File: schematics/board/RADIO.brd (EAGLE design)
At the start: 76 x 76 mm, 50 parts, among them J1 IPX-RADIO, J2 IPX-ANT

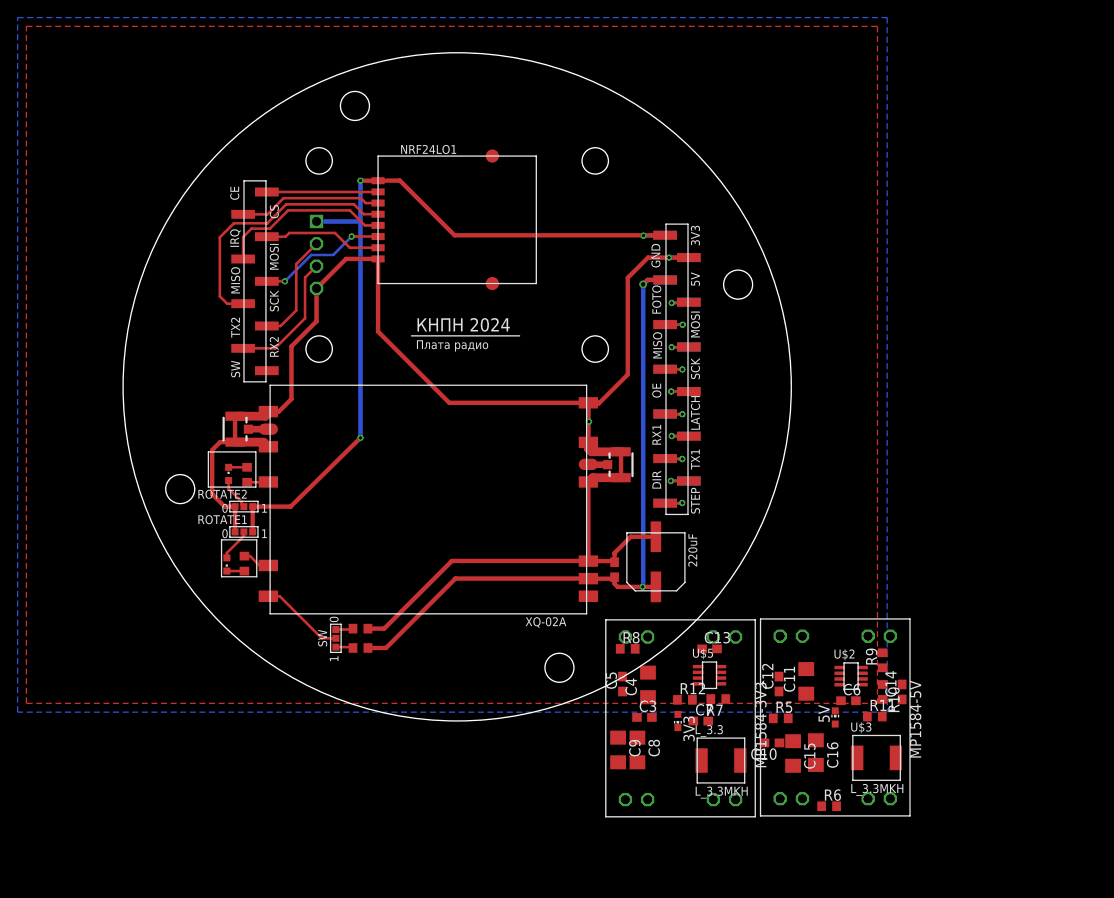
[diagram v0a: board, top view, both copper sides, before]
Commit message: дс дс
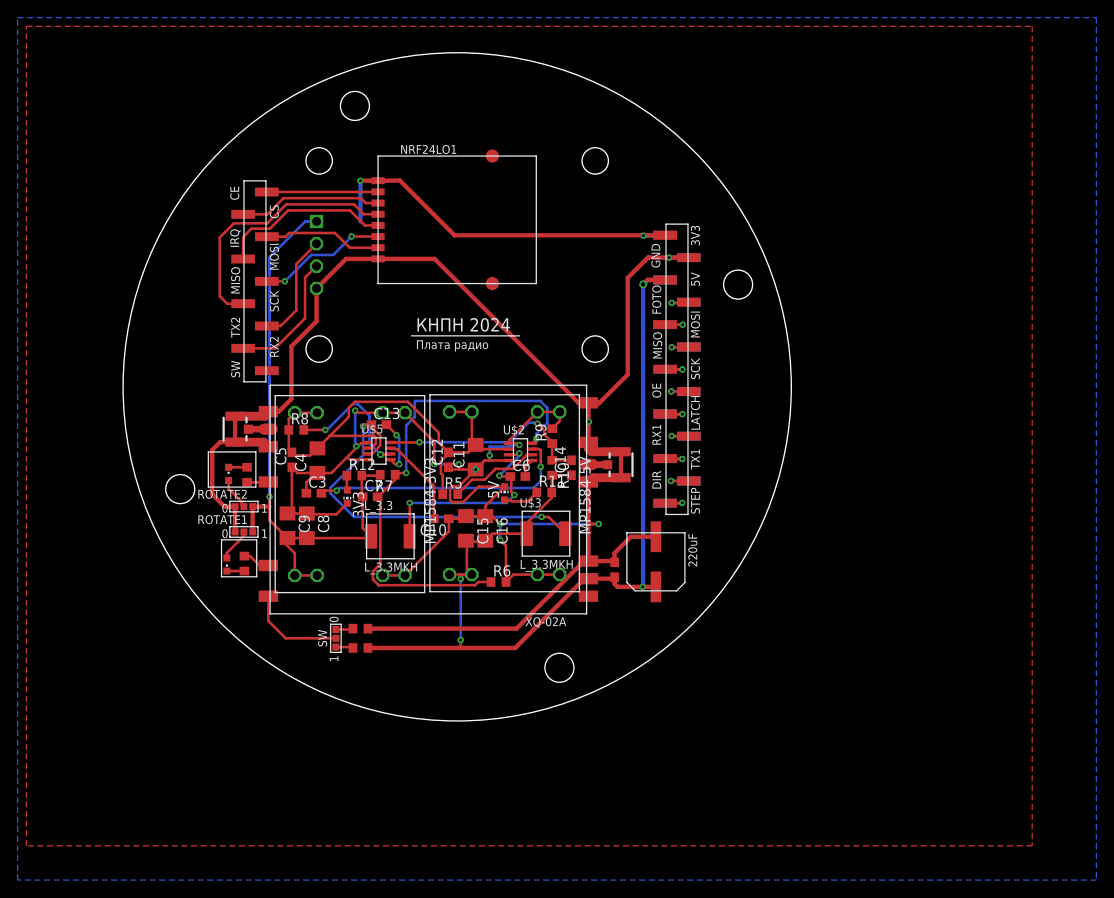
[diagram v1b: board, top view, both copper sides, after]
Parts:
- moved MP1584-3V3 45.4 mm to (37.8, 37.8)
- moved R10 45.4 mm to (60.8, 40.8)
- moved R12 45.4 mm to (38.3, 39.9)
- moved R9 45.4 mm to (60.8, 44.4)
- moved 3V3 45.4 mm to (37.5, 37.5)
- moved 5V 45.4 mm to (55.4, 37.9)
- moved C10 45.4 mm to (48.2, 35.0)
- moved C11 45.4 mm to (52.1, 42.0)
- moved C12 45.4 mm to (49.0, 41.7)
- moved C13 45.4 mm to (41.1, 45.7)
- moved C16 45.4 mm to (53.2, 33.9)
- moved C3 45.4 mm to (33.7, 37.9)
- moved C4 45.4 mm to (34.1, 41.6)
- moved C5 45.4 mm to (31.2, 41.7)
- moved C6 45.4 mm to (56.9, 39.8)
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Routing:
- net GND: track 181.9 -> 309.0 mm, vias 2 -> 12
- net BUS+: track 0.00 -> 57.5 mm
- net N$13: track 0.00 -> 56.6 mm, vias 0 -> 2
- net N$17: track 0.00 -> 43.4 mm, vias 0 -> 2
- net 5V: track 76.8 -> 108.0 mm, vias 2 -> 4
- net N$9: track 0.00 -> 30.1 mm, vias 0 -> 2
- net N$18: track 0.00 -> 24.8 mm, vias 0 -> 2
- net N$12: track 0.00 -> 24.4 mm, vias 0 -> 4
- net 3V3: track 92.3 -> 114.9 mm
- net N$15: track 0.00 -> 15.3 mm, vias 0 -> 3
- net N$14: track 0.00 -> 10.5 mm
- net N$10: track 0.00 -> 10.3 mm
- net N$16: track 0.00 -> 6.32 mm, vias 0 -> 2
- net N$19: track 0.00 -> 4.15 mm
- net N$11: track 0.00 -> 2.14 mm
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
